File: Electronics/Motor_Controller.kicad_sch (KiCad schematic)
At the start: 5 parts, among them U1 RP2040, U4 W25Q32JVZP

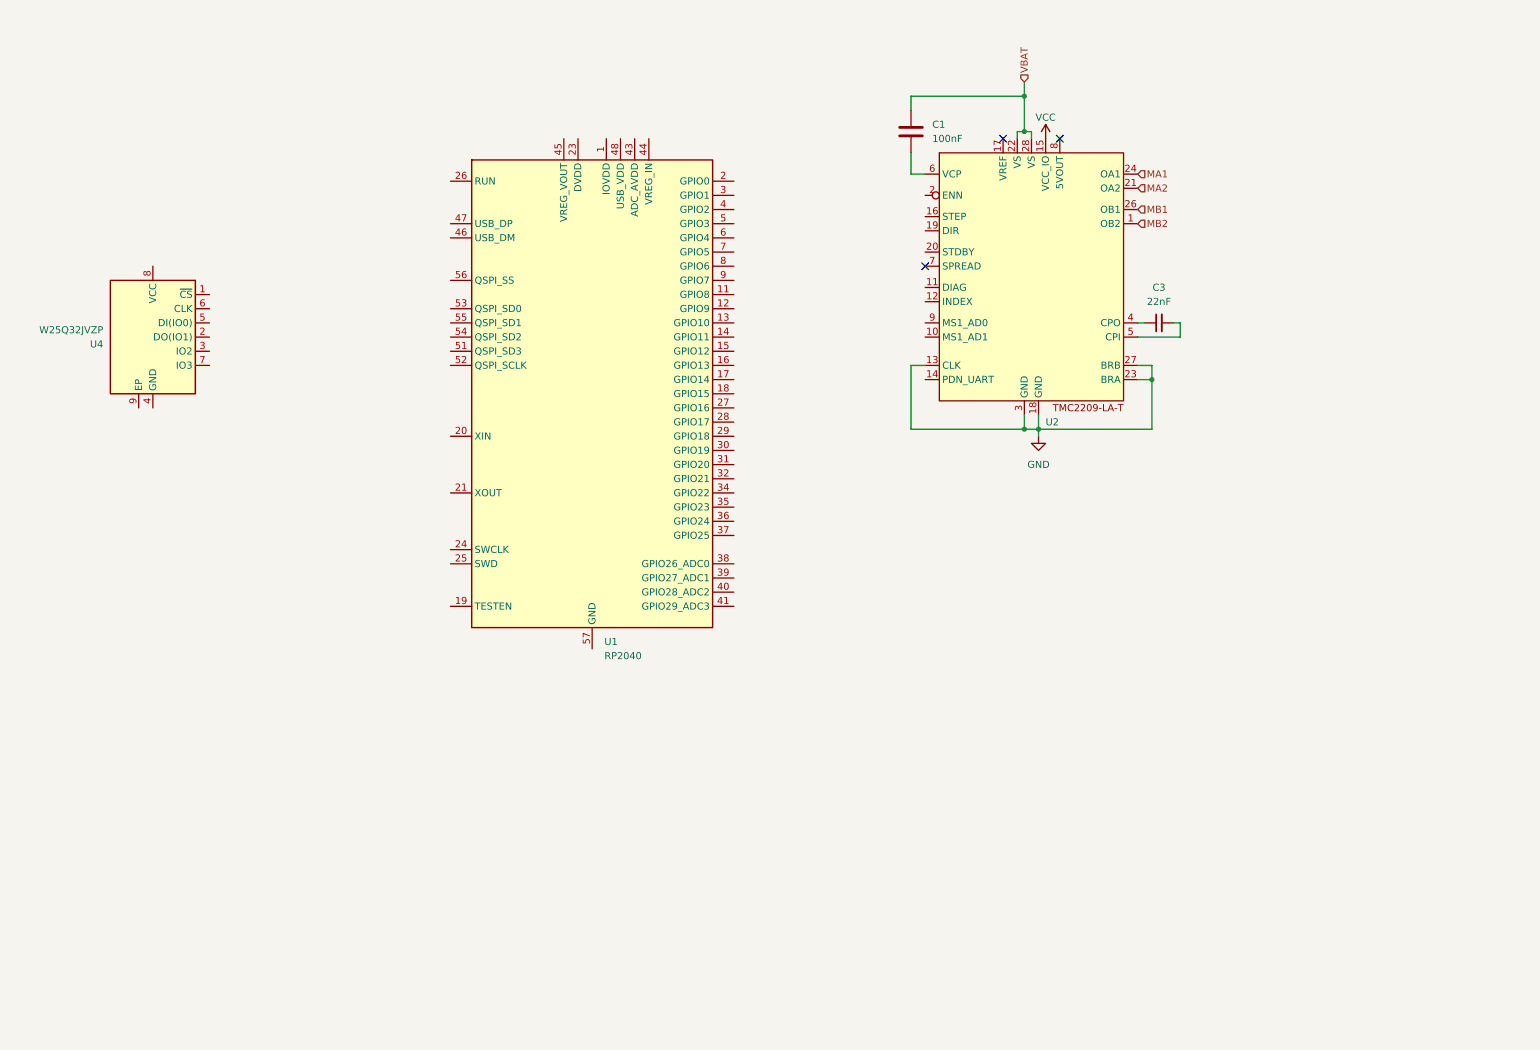
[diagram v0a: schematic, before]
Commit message: motor driver finished!
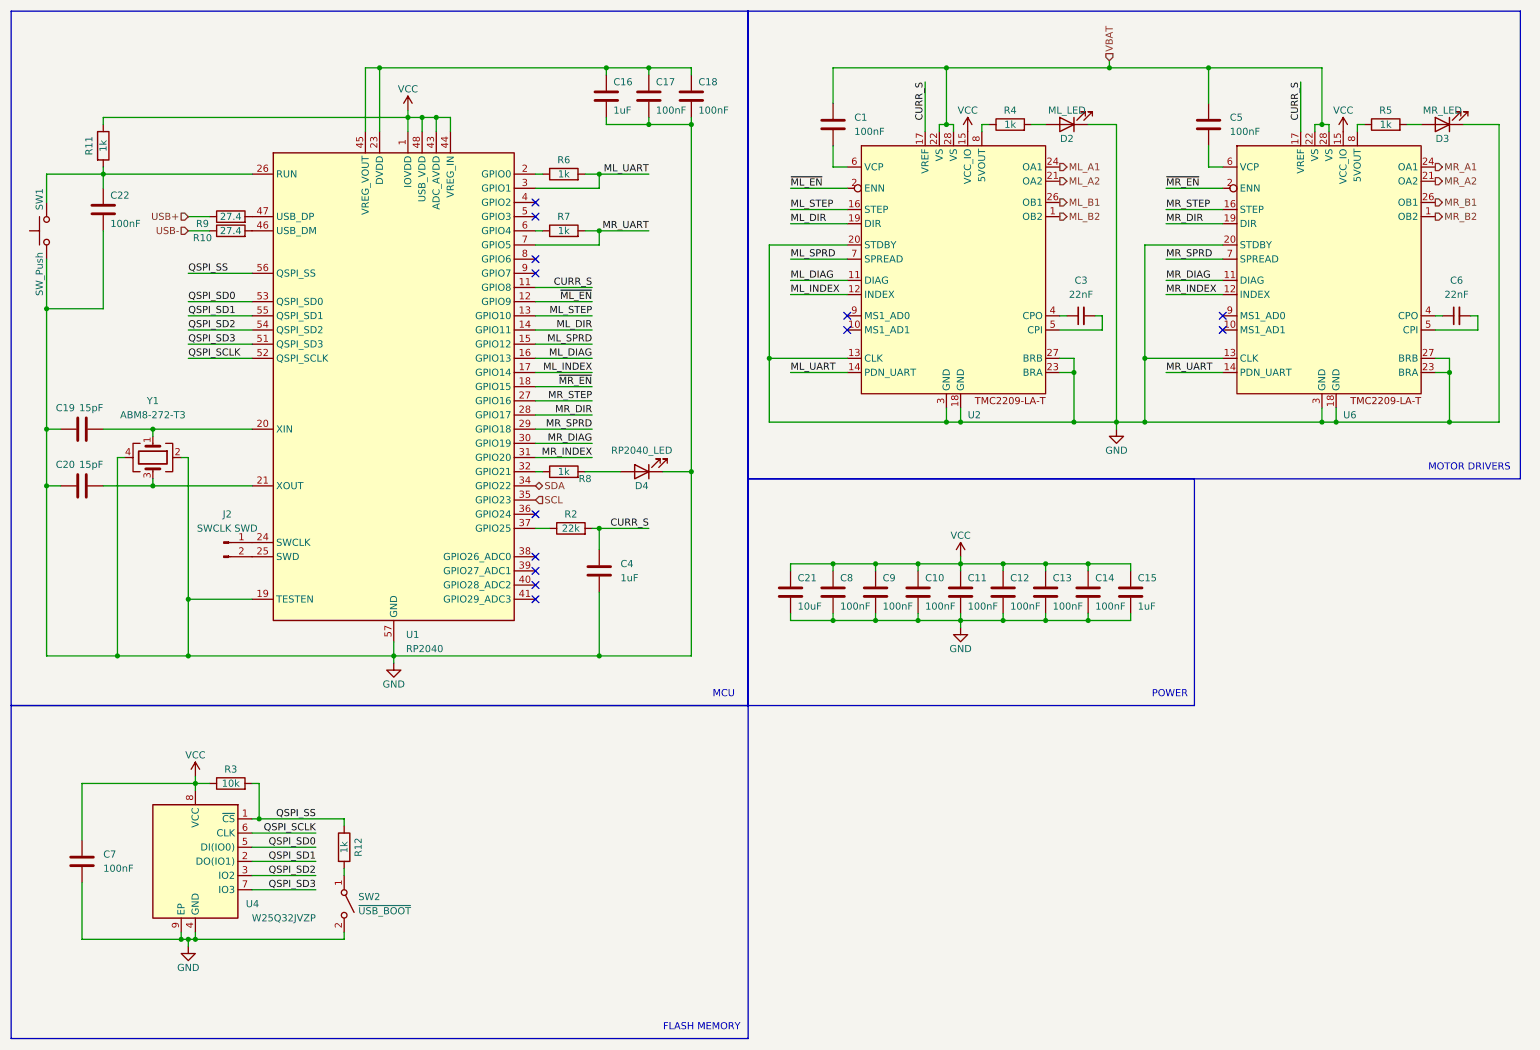
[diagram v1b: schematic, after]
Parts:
- added C10, C11, C12, C13, C14, C17, C18, C22, C5, C7, C8, C9: 100nF, symbol Device:C
- added C15, C16, C4: 1uF, symbol Device:C
- added C19, C20: 15pF, symbol Device:C
- added C21: 10uF, symbol Device:C
- added C6: 22nF, symbol Device:C_Small
- added D2: ML_LED, symbol Device:LED
- added D3: MR_LED, symbol Device:LED
- added D4: RP2040_LED, symbol Device:LED
- added J2: SWCLK SWD, symbol Connector:Conn_01x02_Pin
- added R10, R9: 27.4, symbol Device:R
- added R11, R12, R4, R5, R6, R7, R8: 1k, symbol Device:R
- added R2: 22k, symbol Device:R
- added R3: 10k, symbol Device:R
- added SW1: SW_Push, symbol Switch:SW_Push
- added SW2: ~{USB_BOOT}, symbol Switch:SW_SPST
- added U6: ~, Package_DFN_QFN:QFN-28-1EP_5x5mm_P0.5mm_EP3.75x3.75mm, symbol TMC2209-LA-T:TMC2209-LA-T
- added Y1: ABM8-272-T3, symbol Device:Crystal_GND24
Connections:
- net GND: now also U1.19 (TESTEN), U1.57 (GND), U2.20 (STDBY), U4.4 (GND), U4.9 (EP), C10.2, C11.2, C12.2, C13.2, C14.2, C15.2, C16.2, C17.2, C18.2, C19.1, C20.1, C21.2, C22.2, C4.2, C7.2, C8.2, C9.2, D2.1 (K), D3.1 (K), D4.1 (K), SW1.1, SW2.2 (B), U6.13 (CLK), U6.18 (GND), U6.20 (STDBY), U6.23 (BRA), U6.27 (BRB), U6.3 (GND), Y1.2, Y1.4
- net VBAT: now also C5.1, U6.22 (VS), U6.28 (VS)
- net VCC: now also U1.1 (IOVDD), U1.10 (IOVDD), U1.22 (IOVDD), U1.33 (IOVDD), U1.42 (IOVDD), U1.43 (ADC_AVDD), U1.44 (VREG_IN), U1.48 (USB_VDD), U1.49 (IOVDD), U4.8 (VCC), C10.1, C11.1, C12.1, C13.1, C14.1, C15.1, C21.1, C7.1, C8.1, C9.1, R11.1, R3.1, U6.15 (VCC_IO)
- net ML_DIAG: now reaches U2.11 (DIAG)
- net ML_DIAG: now also U1.16 (GPIO13)
- net ML_INDEX: now reaches U2.12 (INDEX)
- net ML_INDEX: now also U1.17 (GPIO14)
- net ML_UART: now reaches U2.14 (PDN_UART)
- net ML_UART: now also U1.3 (GPIO1), R6.2
- net ML_STEP: now reaches U2.16 (STEP)
- net ML_STEP: now also U1.13 (GPIO10)
- net CURR_S: now reaches U2.17 (VREF)
- net CURR_S: now also U1.11 (GPIO8), C4.1, R2.2, U6.17 (VREF)
- net ML_DIR: now reaches U2.19 (DIR)
- net ML_DIR: now also U1.14 (GPIO11)
- net ~{ML_EN}: now reaches U2.2 (ENN)
- net ~{ML_EN}: now also U1.12 (GPIO9)
- net ML_SPRD: now reaches U2.7 (SPREAD)
- net ML_SPRD: now also U1.15 (GPIO12)
- net at U2.8 (5VOUT): now also R4.1
- net ~{MR_EN}: now reaches U1.18 (GPIO15)
- net ~{MR_EN}: now also U6.2 (ENN)
- net at U1.2 (GPIO0): now also R6.1
- net at U1.20 (XIN): now also C19.2, Y1.1
- net at U1.21 (XOUT): now also C20.2, Y1.3
- net at U1.23 (DVDD), U1.50 (DVDD): now also U1.45 (VREG_VOUT), C16.1, C17.1, C18.1
- net at U1.24 (SWCLK): now also J2.1 (Pin_1)
- net at U1.25 (SWD): now also J2.2 (Pin_2)
- net at U1.26 (RUN): now also C22.1, R11.2, SW1.2
- net MR_STEP: now reaches U1.27 (GPIO16)
- net MR_STEP: now also U6.16 (STEP)
- net MR_DIR: now reaches U1.28 (GPIO17)
- net MR_DIR: now also U6.19 (DIR)
- net MR_SPRD: now reaches U1.29 (GPIO18)
- net MR_SPRD: now also U6.7 (SPREAD)
- net MR_DIAG: now reaches U1.30 (GPIO19)
- net MR_DIAG: now also U6.11 (DIAG)
- net MR_INDEX: now reaches U1.31 (GPIO20)
- net MR_INDEX: now also U6.12 (INDEX)
- net at U1.32 (GPIO21): now also R8.1
- net SDA: now reaches U1.34 (GPIO22)
- net SCL: now reaches U1.35 (GPIO23)
- net at U1.37 (GPIO25): now also R2.1
- net at U1.46 (USB_DM): now also R10.2
- net at U1.47 (USB_DP): now also R9.2
- net QSPI_SD3: now reaches U1.51 (QSPI_SD3)
- net QSPI_SD3: now also U4.7 (IO3)
- net QSPI_SCLK: now reaches U1.52 (QSPI_SCLK)
- net QSPI_SCLK: now also U4.6 (CLK)
- net QSPI_SD0: now reaches U1.53 (QSPI_SD0)
- net QSPI_SD0: now also U4.5 (DI(IO0))
- net QSPI_SD2: now reaches U1.54 (QSPI_SD2)
- net QSPI_SD2: now also U4.3 (IO2)
- net QSPI_SD1: now reaches U1.55 (QSPI_SD1)
- net QSPI_SD1: now also U4.2 (DO(IO1))
- net QSPI_SS: now reaches U1.56 (QSPI_SS)
- net QSPI_SS: now also U4.1 (~{CS}), R12.1, R3.2
- net at U1.6 (GPIO4): now also R7.1
- net MR_UART: now reaches U1.7 (GPIO5)
- net MR_UART: now also R7.2, U6.14 (PDN_UART)
- net MA1 renamed ML_A1
- net MA2 renamed ML_A2
- net MB1 renamed ML_B1
- net MB2 renamed ML_B2
- new net: C6.1, U6.4 (CPO)
- new net: C6.2, U6.5 (CPI)
- new net: C5.2, U6.6 (VCP)
- new net: R5.1, U6.8 (5VOUT)
- new net: R12.2, SW2.1 (A)
- new net: D2.2 (A), R4.2
- new net: D3.2 (A), R5.2
- new net: D4.2 (A), R8.2
- new net MR_A1: U6.24 (OA1)
- new net MR_A2: U6.21 (OA2)
- new net MR_B1: U6.26 (OB1)
- new net MR_B2: U6.1 (OB2)
- new net USB+: R9.1
- new net USB-: R10.1
- no-connect marks 3 -> 13
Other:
- note added: "FLASH MEMORY"
- note added: "MCU"
- note added: "MOTOR DRIVERS"
- note added: "POWER"
- moved on the sheet: C1, C3, U1, U2, U4
